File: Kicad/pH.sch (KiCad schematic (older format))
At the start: 1 part, among them U2 MCP6242

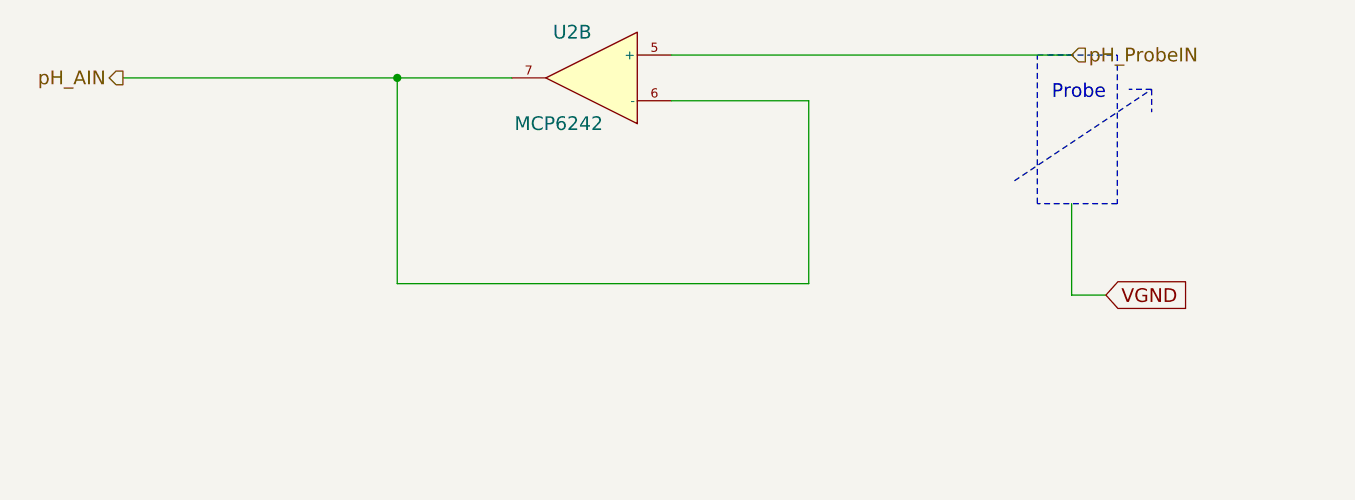
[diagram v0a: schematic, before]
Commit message: layout for Alpha 2
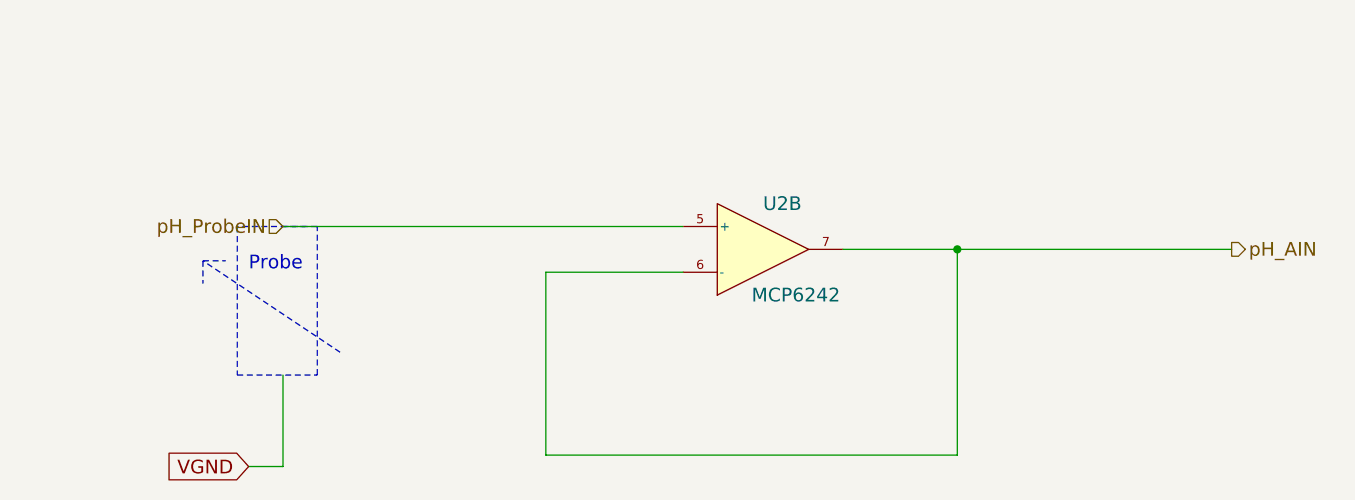
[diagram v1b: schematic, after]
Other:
- moved on the sheet: U2B
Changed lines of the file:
@@
 Sheet 4 11
 Title ""
-Date "29 jan 2015"
+Date "8 feb 2015"
 Rev ""
 Comp ""
@@
 Comment4 ""
 $EndDescr
-Text HLabel 1750 3200 0    60   Output ~ 0
+Text HLabel 6600 3950 2    60   Output ~ 0
 pH_AIN
 Wire Wire Line
-	4150 3100 5900 3100
+	4200 3850 2450 3850
 Wire Wire Line
-	2950 4100 4750 4100
+	5400 4850 3600 4850
 Wire Wire Line
-	4750 4100 4750 3300
+	3600 4850 3600 4050
 Wire Wire Line
-	4750 3300 4150 3300
+	3600 4050 4200 4050
 Wire Wire Line
-	1750 3200 3450 3200
+	6600 3950 4900 3950
 Wire Wire Line
-	2950 4100 2950 3200
-Connection ~ 2950 3200
-Text HLabel 5900 3100 2    60   Input ~ 0
+	5400 4850 5400 3950
+Connection ~ 5400 3950
+Text HLabel 2450 3850 0    60   Input ~ 0
 pH_ProbeIN
-Text Notes 6050 3300 2    60   ~ 0
+Text Notes 2300 4050 0    60   ~ 0
 Probe
 Wire Notes Line
-	5800 3100 6100 3100
+	2550 3850 2250 3850
 Wire Notes Line
-	6100 3750 5750 3750
+	2250 4500 2600 4500
 Wire Notes Line
-	5750 3750 5750 3100
+	2600 4500 2600 3850
 Wire Notes Line
-	5750 3100 5900 3100
+	2600 3850 2450 3850
 Wire Notes Line
-	6100 3100 6100 3750
+	2250 3850 2250 4500
 Wire Notes Line
-	5650 3650 6250 3250
+	2700 4400 2100 4000
 Wire Notes Line
-	6250 3250 6250 3350
+	2100 4000 2100 4100
 Wire Notes Line
-	6250 3250 6150 3250
+	2100 4000 2200 4000
 Wire Wire Line
-	5900 3750 5900 4150
+	2450 4500 2450 4900
 Wire Wire Line
-	5900 4150 6050 4150
-Text GLabel 6050 4150 2    60   Input ~ 0
+	2450 4900 2300 4900
+Text GLabel 2300 4900 0    60   Input ~ 0
 VGND
 $Comp
 L MCP6242 U2
 U 2 1 54906D15
-P 3900 3200
-F 0 "U2" H 4000 3400 60  0000 L CNN
-F 1 "MCP6242" H 3950 3000 60  0000 L CNN
-F 2 "~" H 4000 3200 60  0000 C CNN
-F 3 "~" H 4000 3200 60  0000 C CNN
-	2    3900 3200
-	-1   0    0    -1
+P 4450 3950
+F 0 "U2" H 4550 4150 60  0000 L CNN
+F 1 "MCP6242" H 4500 3750 60  0000 L CNN
+F 2 "~" H 4550 3950 60  0000 C CNN
+F 3 "~" H 4550 3950 60  0000 C CNN
+	2    4450 3950
+	1    0    0    -1
 $EndComp
 $EndSCHEMATC
